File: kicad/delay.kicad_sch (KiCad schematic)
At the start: 58 parts, among them Q1 2N3904, U3 TL074, U4 TL072, U5 PT2399, U6 4020

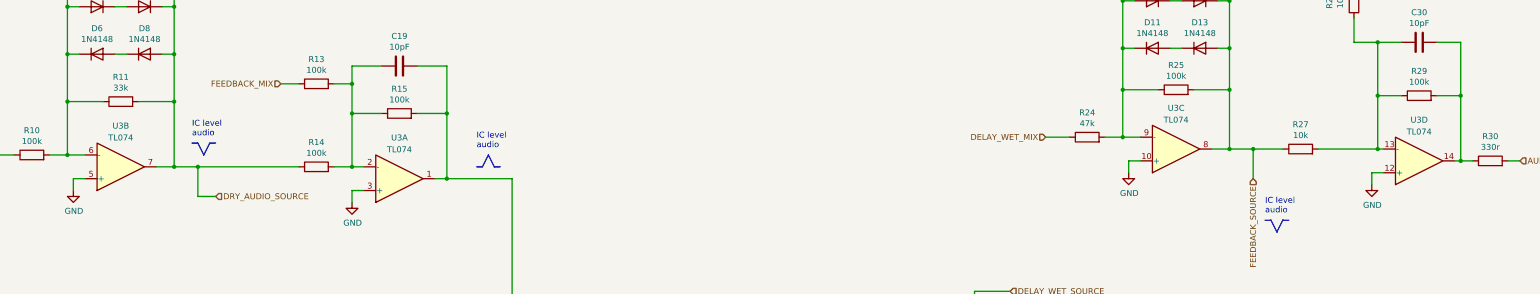
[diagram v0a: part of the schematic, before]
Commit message: initial layout done
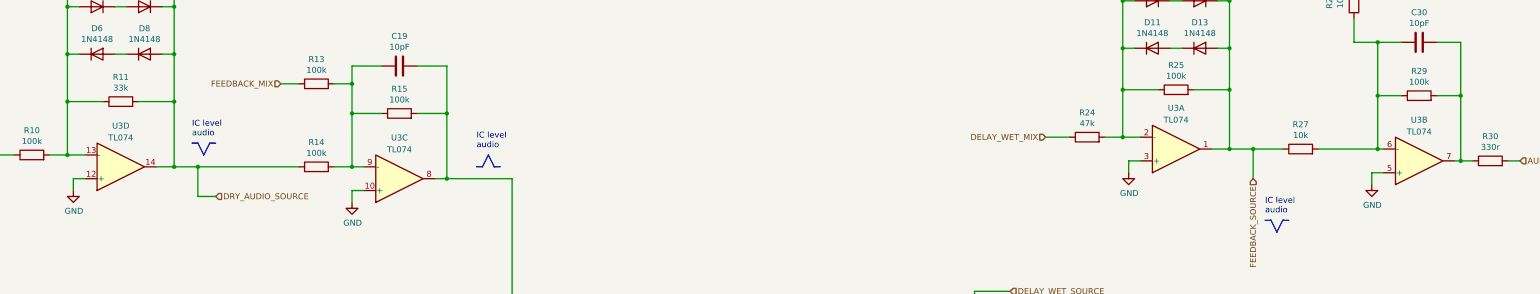
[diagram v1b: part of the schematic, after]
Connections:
- net DRY_AUDIO_SOURCE: now also U3.14; no longer U3.7
- net FEEDBACK_SOURCE: now also U3.1; no longer U3.8
- net at C8.2, D5.2 (A), D6.1 (K)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: now also U3.13 (-); no longer U3.6 (-)
- net at C19.1, C22.1, R15.2: now also U3.8; no longer U3.1
- net at C19.2, R13.2, R14.2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: now also U3.9 (-); no longer U3.2 (-)
- net at C29.2, D10.2 (A), D11.1 (K)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: now also U3.2 (-); no longer U3.9 (-)
- net at C30.1, R29.2, R30.1: now also U3.7; no longer U3.14
- net at C30.2, R27.2, R28.1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: now also U3.6 (-); no longer U3.13 (-)
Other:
- moved on the sheet: U3A, U3B, U3C, U3D
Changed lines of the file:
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@@
     (pin "2")
   )
-  (symbol (lib_id "Amplifier_Operational:TL074") (at 62.23 76.2 0) (mirror x) (unit 2)
-    (in_bom yes) (on_board yes) (fields_autoplaced)
-    (property "Reference" "U3" (id 0) (at 62.23 67.4202 0))
-    (property "Value" "TL074" (id 1) (at 62.23 69.9571 0))
-    (property "Footprint" "rumblesan-standard-parts:DIP-14_W7.62mm_Socket" (id 2) (at 60.96 78.74 0)
-      (effects (font (size 1.27 1.27)) hide)
-    )
-    (property "Datasheet" "http://www.ti.com/lit/ds/symlink/tl071.pdf" (id 3) (at 63.5 81.28 0)
+  (symbol (lib_id "Amplifier_Operational:TL074") (at 340.36 74.93 0) (mirror x) (unit 2)
+    (in_bom yes) (on_board yes) (fields_autoplaced)
+    (property "Reference" "U3" (id 0) (at 340.36 66.1502 0))
+    (property "Value" "TL074" (id 1) (at 340.36 68.6871 0))
+    (property "Footprint" "rumblesan-standard-parts:DIP-14_W7.62mm_Socket" (id 2) (at 339.09 77.47 0)
+      (effects (font (size 1.27 1.27)) hide)
+    )
+    (property "Datasheet" "http://www.ti.com/lit/ds/symlink/tl071.pdf" (id 3) (at 341.63 80.01 0)
       (effects (font (size 1.27 1.27)) hide)
     )
@@
     (pin "2")
   )
-  (symbol (lib_id "Amplifier_Operational:TL074") (at 121.92 78.74 0) (mirror x) (unit 1)
-    (in_bom yes) (on_board yes) (fields_autoplaced)
-    (property "Reference" "U3" (id 0) (at 121.92 69.9602 0))
-    (property "Value" "TL074" (id 1) (at 121.92 72.4971 0))
-    (property "Footprint" "rumblesan-standard-parts:DIP-14_W7.62mm_Socket" (id 2) (at 120.65 81.28 0)
-      (effects (font (size 1.27 1.27)) hide)
-    )
-    (property "Datasheet" "http://www.ti.com/lit/ds/symlink/tl071.pdf" (id 3) (at 123.19 83.82 0)
+  (symbol (lib_id "Amplifier_Operational:TL074") (at 288.29 72.39 0) (mirror x) (unit 1)
+    (in_bom yes) (on_board yes) (fields_autoplaced)
+    (property "Reference" "U3" (id 0) (at 288.29 63.6102 0))
+    (property "Value" "TL074" (id 1) (at 288.29 66.1471 0))
+    (property "Footprint" "rumblesan-standard-parts:DIP-14_W7.62mm_Socket" (id 2) (at 287.02 74.93 0)
+      (effects (font (size 1.27 1.27)) hide)
+    )
+    (property "Datasheet" "http://www.ti.com/lit/ds/symlink/tl071.pdf" (id 3) (at 289.56 77.47 0)
       (effects (font (size 1.27 1.27)) hide)
     )
@@
     (pin "2")
   )
-  (symbol (lib_id "Amplifier_Operational:TL074") (at 340.36 74.93 0) (mirror x) (unit 4)
-    (in_bom yes) (on_board yes) (fields_autoplaced)
-    (property "Reference" "U3" (id 0) (at 340.36 66.1502 0))
-    (property "Value" "TL074" (id 1) (at 340.36 68.6871 0))
-    (property "Footprint" "rumblesan-standard-parts:DIP-14_W7.62mm_Socket" (id 2) (at 339.09 77.47 0)
-      (effects (font (size 1.27 1.27)) hide)
-    )
-    (property "Datasheet" "http://www.ti.com/lit/ds/symlink/tl071.pdf" (id 3) (at 341.63 80.01 0)
+  (symbol (lib_id "Amplifier_Operational:TL074") (at 62.23 76.2 0) (mirror x) (unit 4)
+    (in_bom yes) (on_board yes) (fields_autoplaced)
+    (property "Reference" "U3" (id 0) (at 62.23 67.4202 0))
+    (property "Value" "TL074" (id 1) (at 62.23 69.9571 0))
+    (property "Footprint" "rumblesan-standard-parts:DIP-14_W7.62mm_Socket" (id 2) (at 60.96 78.74 0)
+      (effects (font (size 1.27 1.27)) hide)
+    )
+    (property "Datasheet" "http://www.ti.com/lit/ds/symlink/tl071.pdf" (id 3) (at 63.5 81.28 0)
       (effects (font (size 1.27 1.27)) hide)
     )
@@
     (pin "2")
   )
-  (symbol (lib_id "Amplifier_Operational:TL074") (at 288.29 72.39 0) (mirror x) (unit 3)
-    (in_bom yes) (on_board yes) (fields_autoplaced)
-    (property "Reference" "U3" (id 0) (at 288.29 63.6102 0))
-    (property "Value" "TL074" (id 1) (at 288.29 66.1471 0))
-    (property "Footprint" "rumblesan-standard-parts:DIP-14_W7.62mm_Socket" (id 2) (at 287.02 74.93 0)
-      (effects (font (size 1.27 1.27)) hide)
-    )
-    (property "Datasheet" "http://www.ti.com/lit/ds/symlink/tl071.pdf" (id 3) (at 289.56 77.47 0)
-      (effects (font (size 1.27 1.27)) hide)
-    )
+  (symbol (lib_id "Amplifier_Operational:TL074") (at 121.92 78.74 0) (mirror x) (unit 3)
+    (in_bom yes) (on_board yes) (fields_autoplaced)
+    (property "Reference" "U3" (id 0) (at 121.92 69.9602 0))
+    (property "Value" "TL074" (id 1) (at 121.92 72.4971 0))
+    (property "Footprint" "rumblesan-standard-parts:DIP-14_W7.62mm_Socket" (id 2) (at 120.65 81.28 0)
+      (effects (font (size 1.27 1.27)) hide)
+    )
+    (property "Datasheet" "http://www.ti.com/lit/ds/symlink/tl071.pdf" (id 3) (at 123.19 83.82 0)
+      (effects (font (size 1.27 1.27)) hide)
+    )
